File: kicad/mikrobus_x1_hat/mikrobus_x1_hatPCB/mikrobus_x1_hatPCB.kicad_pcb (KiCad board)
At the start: 2 copper layers, 65 x 56.5 mm, 6 parts, among them IC1 MIKROE-924, J1 RPi_GPIO

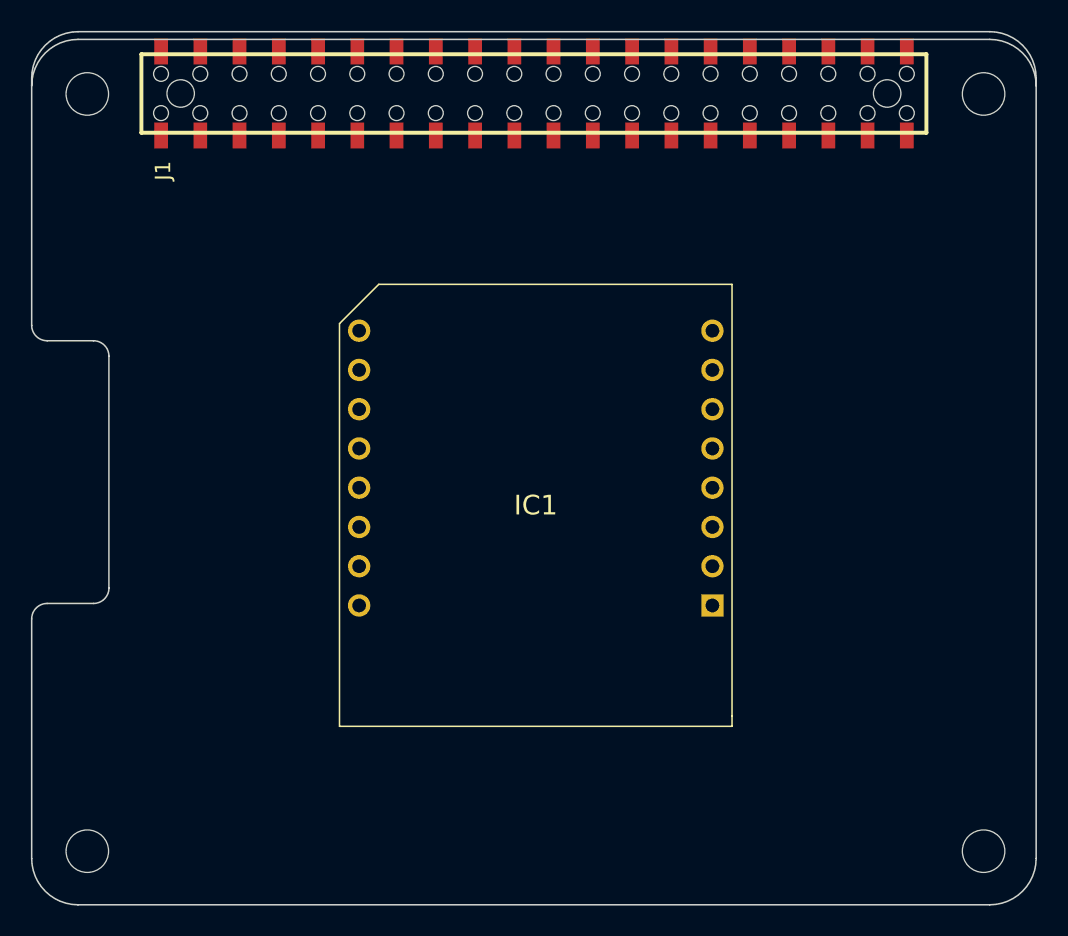
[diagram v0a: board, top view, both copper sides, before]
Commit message: pcb routing initiated
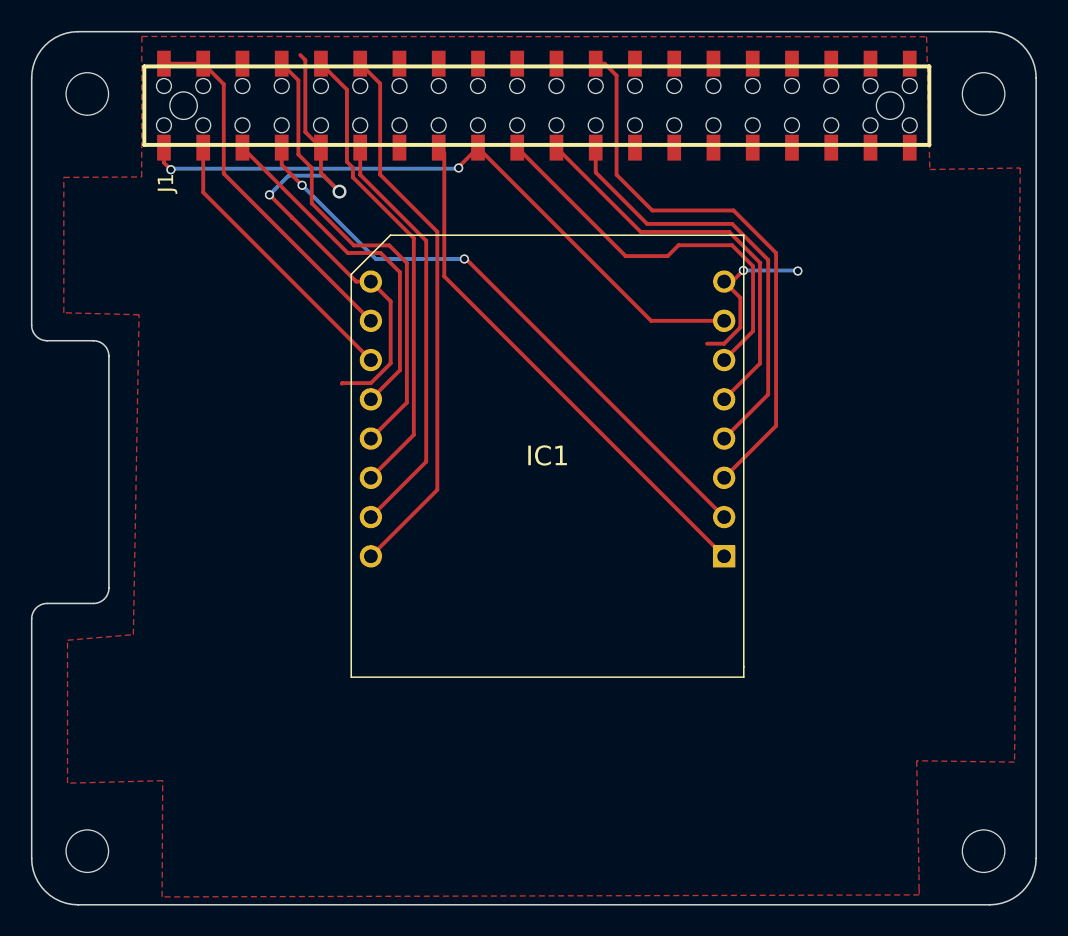
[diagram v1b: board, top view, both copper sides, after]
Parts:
- moved IC1 3.27 mm to (160.0, 104.5)
- moved J1 0.81 mm to (147.9, 75.3)
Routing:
- net GND: track 0.00 -> 44.9 mm, vias 0 -> 4
- net 3V3: track 0.00 -> 42.7 mm, vias 0 -> 2
- net Net-(IC1-RST): track 0.00 -> 39.2 mm, vias 0 -> 2
- net Net-(IC1-CS): track 0.00 -> 36.4 mm
- net Net-(IC1-PWM): track 0.00 -> 35.7 mm
- net Net-(IC1-AN): track 0.00 -> 34.1 mm
- net Net-(IC1-RX): track 0.00 -> 30.4 mm
- net Net-(IC1-TX): track 0.00 -> 29.9 mm
- net Net-(IC1-SCK): track 0.00 -> 27.8 mm
- net Net-(IC1-INT): track 0.00 -> 27.2 mm
- net Net-(IC1-MISO): track 0.00 -> 26.1 mm
- net Net-(IC1-MOSI): track 0.00 -> 25.9 mm
- net 5V: track 0.00 -> 23.7 mm
- net Net-(IC1-SCL): track 0.00 -> 22.5 mm
- net Net-(IC1-SDA): track 0.00 -> 18.2 mm
- added copper zone on F.Cu, net GND
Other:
- outline, holes or cut-outs redrawn
